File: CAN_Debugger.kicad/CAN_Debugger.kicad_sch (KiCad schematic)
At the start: 72 parts, among them J1 Conn_01x02, J2 Conn_01x04_MountingPin, J4 Conn_01x16_Socket, J7 CAN, J8 CAN, J9 CAN, Q1 AO3400A, SW1 SW_Push, SW2 SW_Push, SW3 SW_Push, U1 STM32F103C8Tx, U2 RY8411, U3 RS3236, U5 TJA1042T-3, Y1 Crystal

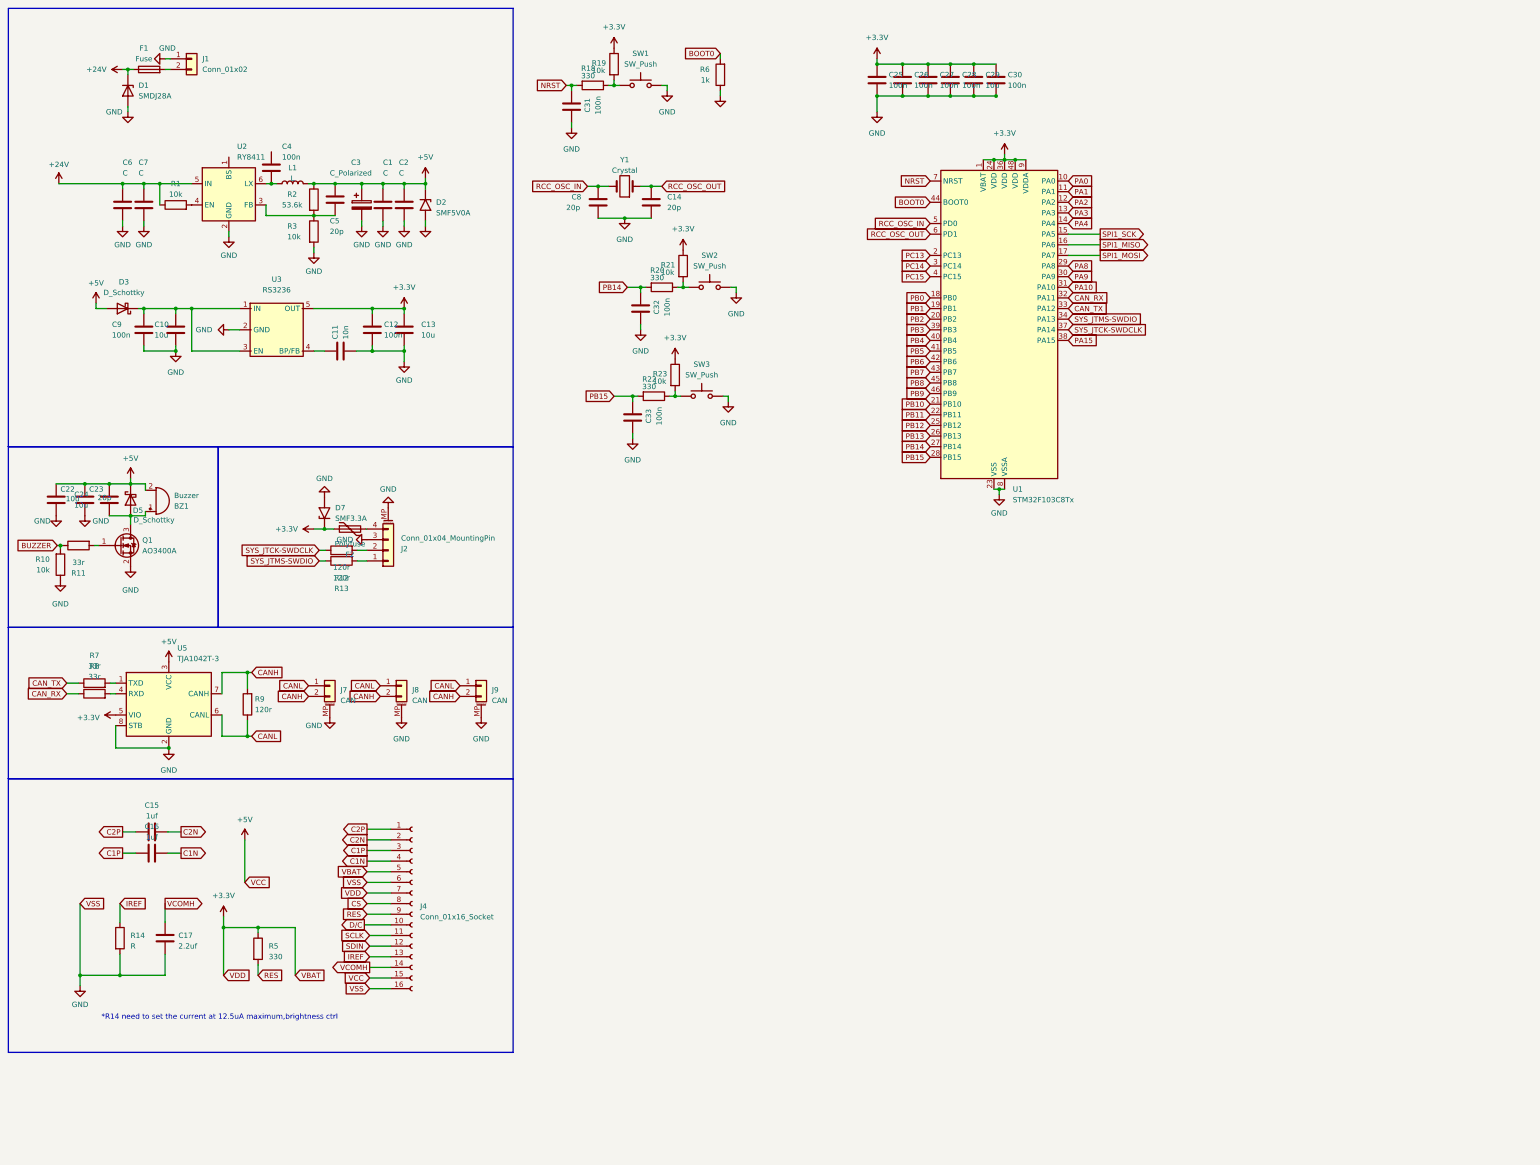
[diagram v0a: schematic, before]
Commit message: Kicad Schematic done
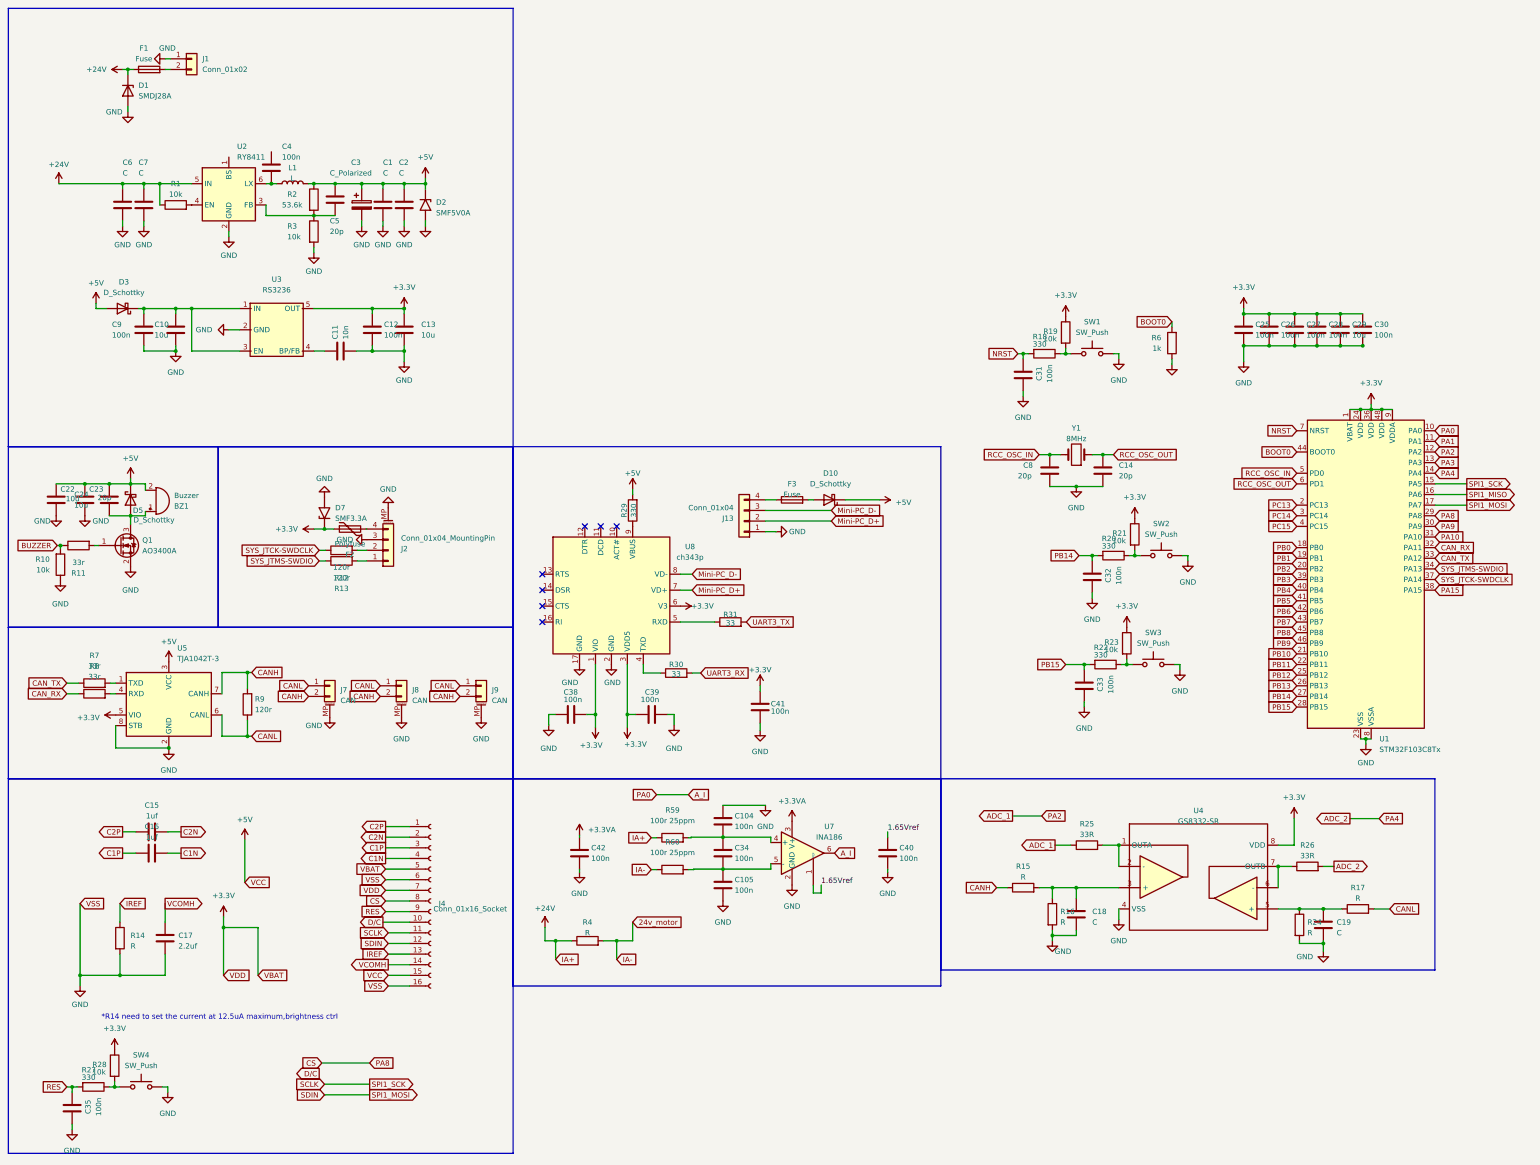
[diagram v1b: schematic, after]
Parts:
- removed R5: 330, symbol Device:R
- added C104, C105, C34, C35, C38, C39, C40, C41, C42: 100n, Capacitor_SMD:C_0603_1608Metric, symbol Device:C
- added C18, C19: C, symbol Device:C
- added D10: D_Schottky, Diode_SMD:D_SMF, symbol Device:D_Schottky
- added F3: Fuse, Fuse:Fuse_1206_3216Metric, symbol Device:Fuse
- added J13: Conn_01x04, ENTERPRIZE2024_internal_JYC_v0:Micro USB, symbol Connector_Generic:Conn_01x04
- added R15, R16, R17, R24, R4: R, symbol Device:R
- added R25, R26: 33R, symbol Device:R
- added R27, R29: 330, Resistor_SMD:R_0603_1608Metric, symbol Device:R
- added R28: 10k, Resistor_SMD:R_0603_1608Metric, symbol Device:R
- added R30, R31: 33, Resistor_SMD:R_0603_1608Metric, symbol Device:R
- added R59, R60: 100r 25ppm, Resistor_SMD:R_0603_1608Metric, symbol Device:R
- added SW4: SW_Push, Button_Switch_SMD:SW_SPST_TL3342, symbol Switch:SW_Push
- added U4: GS8332-SR, symbol 0_RM2023:GS8332-SR
- added U7: INA186, Package_TO_SOT_SMD:SOT-363_SC-70-6, symbol Amplifier_Current:INA199xxDCK
- added U8: ch343p, ENTERPRIZE2024_internal_JYC_v0:QFN17, symbol 0_RM2023:ch343p
- Y1: value Crystal -> 8MHz
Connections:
- net PA8 is gone; now on net CS: U1.29 (PA8)
- net SPI1_MOSI is gone; now on net SDIN: U1.17 (PA7)
- net SPI1_SCK is gone; now on net SCLK: U1.15 (PA5)
- net +24V: now also R4.1, R59.1
- net +3.3V: now also C38.1, C39.1, C41.1, R28.1, U4.8 (VDD), U8.1 (VIO), U8.3 (VDD5), U8.6 (V3)
- net +5V: now also D10.1 (K), R29.2
- net CANH: now also R15.1
- net CANL: now also R17.2
- net GND: now also C104.1, C105.2, C18.2, C19.2, C35.1, C38.2, C39.2, C40.2, C41.2, C42.2, J13.1 (Pin_1), R16.2, R24.2, SW4.2, U4.4 (VSS), U7.2 (GND), U8.17 (GND), U8.2 (GND)
- net RES: now also C35.2, R27.2
- net PA0 renamed A_I
- net A_I: now also U7.6
- net PA2 renamed ADC_1
- net ADC_1: now also R25.1
- net PA4 renamed ADC_2
- net ADC_2: now also R26.2
- new net: C104.2, C34.1, R59.2, U7.4 (+)
- new net: R27.1, R28.2, SW4.1
- new net: F3.1, J13.4 (Pin_4)
- new net: R31.1, U8.5 (RXD)
- new net: C19.1, R17.1, R24.1, U4.5 (+)
- new net: C18.1, R15.2, R16.1, U4.3 (+)
- new net: R25.2, U4.1 (OUTA), U4.2 (-)
- new net: R26.1, U4.6 (-), U4.7 (OUTB)
- new net: D10.2 (A), F3.2
- new net: C105.1, C34.2, R60.2, U7.5 (-)
- new net: R30.1, U8.4 (TXD)
- new net: R29.1, U8.9 (VBUS)
- new net +3.3VA: C42.1, U7.3 (V+)
- new net 1.65Vref: C40.1, U7.1 (REF)
- new net 24v_motor: R4.2, R60.1
- new net Mini-PC_D+: J13.2 (Pin_2), U8.7 (VD+)
- new net Mini-PC_D-: J13.3 (Pin_3), U8.8 (VD-)
- new net UART3_RX: R30.2
- new net UART3_TX: R31.2
- no-connect marks 0 -> 7
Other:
- moved on the sheet: C14, C25, C26, C27, C28, C29, C30, C31, C32, C33, C8, J4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
